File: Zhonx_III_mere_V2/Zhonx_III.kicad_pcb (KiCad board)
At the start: 2 copper layers, 70 x 97 mm, 133 parts, among them K1 L_Motor, K2 R_Motor, K3 USART, P1 JTAG, Q1 FDV301N, Q2 FDV301N, U1 MCP73213, U10 BSL214N, U11 BSL214N, U12 24LC64T, U14 STM32F405RGT6, U16 Line_1, U17 Line_2, U18 Line_3, U19 Line_4, U2 A3918, U20 Line_5, U3 A3918, U4 LTC2955CTS8-2, U5 SIB911DK, U6 SI1551DL, U7 LM2940, U8 MCP1700, U9 MCP1700, X1 16MHz

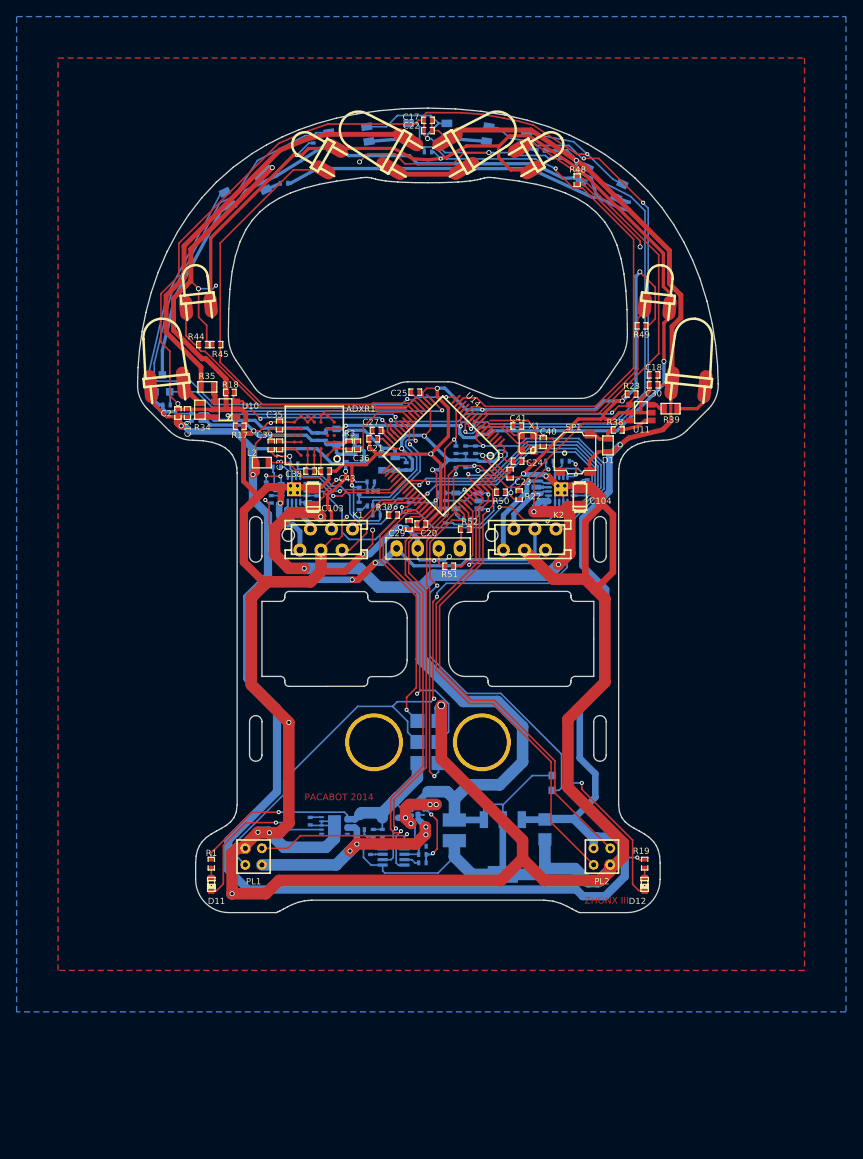
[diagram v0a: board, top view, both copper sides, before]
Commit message: Add ZHONX_III V2
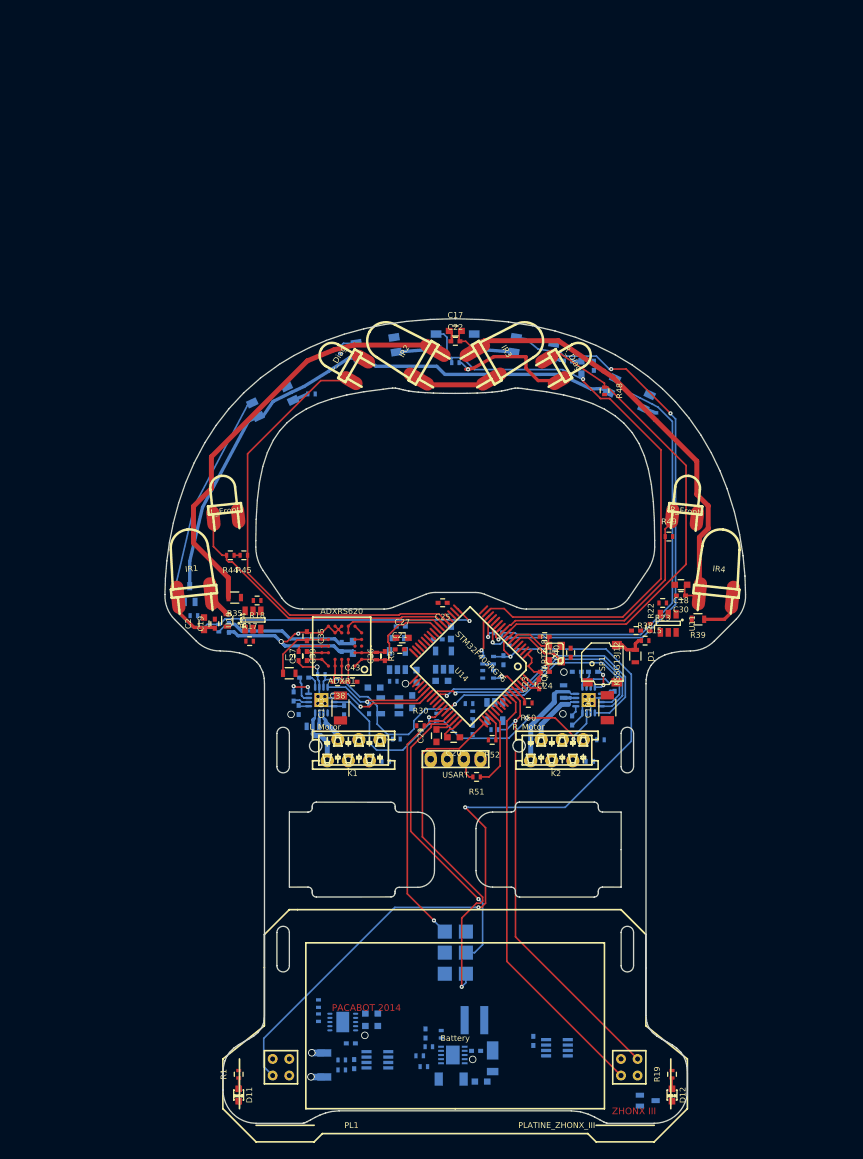
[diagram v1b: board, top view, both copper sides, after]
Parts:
- removed C100: 100uF, SM1210_Capa
- removed C101: 100uF, SM1206_Capa
- added C46: 2,2uF, Capacitors_SMD:C_0603, B.Cu at (111.0, 178.4)
- added C47: 330pF, Capacitors_SMD:C_0402, B.Cu at (104.3, 172.6)
- added C48: 0,47uF, Capacitors_SMD:C_0402, B.Cu at (110.4, 174.7)
- added C49: 0,47uF, Capacitors_SMD:C_0402, B.Cu at (101.3, 123.5)
- added C50: 0,47uF, Capacitors_SMD:C_0402, B.Cu at (105.8, 125.1)
- added C51: 0,47uF, Capacitors_SMD:C_0402, B.Cu at (97.5, 133.5)
- added C52: 10uF, Capacitors_SMD:C_0603, B.Cu at (101.1, 124.9)
- added C53: 10uF, Capacitors_SMD:C_0603, B.Cu at (107.4, 124.3)
- added C54: 10uF, Capacitors_SMD:C_0603, B.Cu at (98.1, 130.9)
- added C55: 33uF, Capacitors_SMD:C_1206, B.Cu at (107.4, 178.1)
- added L1: 2,2uH, ZHONX:XFL4020, B.Cu at (110.2, 171.0)
- added R36: 47K, Resistors_SMD:R_0402, B.Cu at (103.6, 175.3)
- added R37: 0.1 SHNT, Resistors_SMD:R_1206, B.Cu at (92.1, 176.4)
- added R40: 2,2K, Resistors_SMD:R_0402, B.Cu at (99.5, 139.8)
- added R41: 2,2K, Resistors_SMD:R_0402, B.Cu at (124.1, 139.8)
- added R42: 2,2K, Resistors_SMD:R_0402, B.Cu at (100.8, 137.1)
- added R43: 2,2K, Resistors_SMD:R_0402, B.Cu at (125.4, 137.2)
- ADXR1: footprint ADXRS620 -> ZHONX:ADXRS620
- C1, C17, C18, C2, C20, C26, C27, C29, C31, C9: footprint SM0402_ZHONX -> Capacitors_SMD:C_0603
- C10, C11, C12, C13, C14, C19, C21, C22, C23, C24, C25, C28, C3, C30, C32, C33, C35, C37, C38, C39, C4, C40, C41, C43, C44, C45, C5, C6, C7, C8: footprint SM0402_ZHONX -> Capacitors_SMD:C_0402
- C103, C104: footprint SM1206_Capa -> Capacitors_SMD:C_1206
- C15: value 0,1uF -> 10nF; footprint SM0402_ZHONX -> Capacitors_SMD:C_0402; moved to F.Cu
- C16: value 0,1uF -> 2,2uF; footprint SM0402_ZHONX -> Capacitors_SMD:C_0603
- C34: value 1uF -> 2.2uF; footprint SM0402_ZHONX -> Capacitors_SMD:C_0603
- C36: value 22nF -> 2,2nF; footprint SM0402_ZHONX -> Capacitors_SMD:C_0402
- C42: value 10uF -> 2.2uF; footprint SM0603_Capa -> Capacitors_SMD:C_0603
- D1: footprint SM0603 -> Resistors_SMD:R_0603
- D11: value Bleue -> BLUE; footprint LED-0603 -> ZHONX:LED-0603-DVB
- D12: value Blanc -> GREEN; footprint LED-0603 -> ZHONX:LED-0603-DVB
- IR1: footprint IR_LF -> ZHONX:IR_LF
- IR2: footprint IR_LD -> ZHONX:IR_LD
- IR3: footprint IR_RD -> ZHONX:IR_RD
- IR4: footprint IR_RF -> ZHONX:IR_RF
- K1, K2: footprint Connecteur_Moteur_Zhonx -> ZHONX:Connecteur_Moteur_Zhonx
- K3: footprint Conn_Serial_Zhonx -> ZHONX:Conn_Serial_Zhonx
- L2: value 10uH -> BEAD; footprint SM0603 -> Resistors_SMD:R_0603
- P1: footprint Zhonx_III_JTAG -> ZHONX:Zhonx_III_JTAG
- PL1: footprint Platine_Zhonx_III -> ZHONX:Platine_Zhonx_III
- Q1, Q2: value FDV301N -> BSS138; footprint SOT23GDS -> SMD_Packages:SOT-323
- R1: value 3,3K -> 620; footprint SM0402_ZHONX -> Resistors_SMD:R_0402
- R10, R11, R13, R14, R15, R17, R18, R2, R20, R21, R23, R24, R25, R26, R29, R30, R31, R32, R33, R44, R45, R48, R49, R50, R51, R52, R7, R8, R9: footprint SM0402_ZHONX -> Resistors_SMD:R_0402
- R12: value 100K -> 23,7K; footprint SM0402_ZHONX -> Resistors_SMD:R_0402
- R16: value 10K -> 47K; footprint SM0402_ZHONX -> Resistors_SMD:R_0402
- R19: value 820 -> 470; footprint SM0402_ZHONX -> Resistors_SMD:R_0402
- R22: value 47K -> 1M; footprint SM0402_ZHONX -> Resistors_SMD:R_0402
- R27, R28: value 0,2 -> 0,2 603; footprint SM0603_ZHONX -> Resistors_SMD:R_0603
- R3: value 90K -> 90.9K 1%; footprint SM0402_ZHONX -> Resistors_SMD:R_0402
- R34, R39: value 12 -> 10 1W; footprint SM0603_ZHONX -> Resistors_SMD:R_0603
- R35: value 2,8 -> 2,2 2W; footprint SM0603_ZHONX -> Resistors_SMD:R_0603
- R38: value 100 -> 0; footprint SM0402_ZHONX -> Resistors_SMD:R_0402
- R4: value 1M -> 10; footprint SM0402_ZHONX -> Resistors_SMD:R_0402
- R5: value 1M -> 6.2K; footprint SM0402_ZHONX -> Resistors_SMD:R_0402
- R58, R67: value 220 -> 82; footprint SM0402_ZHONX -> Resistors_SMD:R_0402
- R6: value 100K -> 10; footprint SM0402_ZHONX -> Resistors_SMD:R_0402
- R64: value 33 -> 22; footprint SM0402_ZHONX -> Resistors_SMD:R_0402
- SCH1: value BAT60 -> DFLS240; footprint SOD323 -> ZHONX:PowerDI-123
- SP1: footprint Buzzer_KSSG13J12 -> ZHONX:Buzzer_KSSG13J12
- U1: footprint MCP73213 -> ZHONX:MCP73213
- U10, U11: footprint SOT23_6 -> Housings_SOT-23_SOT-143_TSOT-6:SOT-23-6
- U12: footprint SOT23-5 -> Housings_SOT-23_SOT-143_TSOT-6:SOT-23-5
- U14: footprint TQFP_64 -> ZHONX:TQFP_64
- U16, U17, U18, U19, U20: footprint QRE1113GR -> ZHONX:QRE1113GR
- U2: value A3918 -> A3918_L; footprint QFN16_Termal_Pad -> ZHONX:QFN16_Termal_Pad
- U3: value A3918 -> A3918_R; footprint QFN16_Termal_Pad -> ZHONX:QFN16_Termal_Pad
- U4: value LTC2955CTS8-2 -> LTC2955CTS8-1; footprint LTC2955 -> ZHONX:LTC2955
- U5: value SIB911DK -> INA219; footprint SC75-6L -> ZHONX:LTC2955
- U6: value SI1551DL -> LT1761-5; footprint SC70 -> Housings_SOT-23_SOT-143_TSOT-6:SOT-23-5
- U7: value LM2940 -> LT1761-3.3; footprint SOT223 -> Housings_SOT-23_SOT-143_TSOT-6:SOT-23-5
- U8: value MCP1700 -> LT1761-3.3; footprint SOT23 -> Housings_SOT-23_SOT-143_TSOT-6:SOT-23-5
- U9: value MCP1700 -> LT3684; footprint SOT23 -> ZHONX:DFN-10
- X1: value 16MHz -> QUARTZ_8Z; footprint Quartz_8Z-16MHz -> ZHONX:Quartz_8Z-16MHz
- moved U9 75.7 mm to (107.6, 175.2), turned to 270 degrees
- moved R16 69.8 mm to (104.1, 176.6), turned to 0 degrees
- moved R4 67.0 mm to (94.2, 177.0)
- moved R15 65.7 mm to (104.7, 174.2), turned to 180 degrees
- moved R5 63.2 mm to (91.4, 169.0), turned to 270 degrees
- moved C15 40.7 mm to (129.7, 124.0), turned to 180 degrees
- moved Q2 39.7 mm to (131.1, 180.7)
- moved C14 35.2 mm to (95.7, 176.3), turned to 90 degrees
- moved SCH1 31.4 mm to (112.4, 175.5), turned to 90 degrees
- moved U5 30.7 mm to (98.5, 176.1), turned to 90 degrees
- moved U4 30.3 mm to (120.2, 174.7)
- moved C11 30.2 mm to (117.3, 173.5)
- moved C34 29.7 mm to (106.3, 130.1), turned to 180 degrees
- moved U8 29.4 mm to (100.0, 133.1), turned to 180 degrees
- moved C42 28.7 mm to (102.7, 132.6)
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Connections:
- net +5VA renamed +5VADC
- C10 pad 1: GND -> +3.3VADC
- C10 pad 2: N-000003 -> GND
- C14 pad 1: +8V -> Net-(C14-Pad1)
- C14 pad 2: GND -> Net-(C14-Pad2)
- C15 pad 1: +5V -> Net-(C15-Pad1)
- C15 pad 2: GND -> PIEZZO
- C16 pad 1: +3.3V -> +8V
- C17 pad 2: +5V -> +4.5V
- C18 pad 1: +5V -> +4.5V
- C19 pad 1: +5V -> +4.5V
- C2 pad 1: +5V -> +4.5V
- C22 pad 2: +5V -> +4.5V
- C30 pad 1: +5V -> +4.5V
- C31 pad 1: +5V -> +4.5V
- C32 pad 1: +5V -> +4.5V
- C34 pad 1: +5V -> GND
- C34 pad 2: GND -> +5V
- C42 pad 1: +3.3V -> GND
- C42 pad 2: GND -> +4.5V
- C9 pad 1: +BATT -> GND
- C9 pad 2: GND -> +8V
- D1 pad 2: +5V -> +4.5V
- D12 pad 2: N-0000059 -> Net-(D12-Pad2)
- IR1 pad 1: +5V -> +4.5V
- IR3 pad 1: +5V -> +4.5V
- IR4 pad 1: +5V -> +4.5V
- K1 pad 5: L_ENC_B -> Net-(K1-Pad5)
- K1 pad 6: L_ENC_A -> Net-(K1-Pad6)
- K2 pad 5: R_ENC_A -> Net-(K2-Pad5)
- K2 pad 6: R_ENC_B -> Net-(K2-Pad6)
- K3 pad 4: +5V -> +4.5V
- P1 pad 4: NSRST -> PA13/JTMS-SWO
- PL1 pad 5: +5V -> +4.5V
- PL1 pad 8: GND -> WKUP
- R11 pad 2: N-00000103 -> Net-(R11-Pad2)
- R12 pad 1: N-000005 -> Net-(R12-Pad1)
- R12 pad 2: N-0000012 -> GND
- R15 pad 1: TEST_BAT -> Net-(R15-Pad1)
- R15 pad 2: N-0000093 -> Net-(C47-Pad1)
- R16 pad 1: GND -> Net-(R16-Pad1)
- R16 pad 2: TEST_BAT -> +4.5V
- R19 pad 2: +5V -> +4.5V
- R22 pad 1: PIEZZO -> Net-(C15-Pad1)
- R4 pad 1: GND -> Net-(C14-Pad1)
- R4 pad 2: GET_BAT_ADC -> +BATT
- R5 pad 1: +8V -> FAST_CHARGE
- R5 pad 2: N-0000067 -> Net-(R11-Pad2)
- R58 pad 2: +5V -> +4.5V
- R6 pad 1: +9V -> Net-(C14-Pad2)
- R6 pad 2: GND -> +8V
- R64 pad 2: +5V -> +4.5V
- R67 pad 2: +5V -> +4.5V
- R9 pad 1: N-000003 -> EN_PW_ADC
- R9 pad 2: N-000005 -> GND
- SCH1 pad 1: +9V -> GND
- SCH1 pad 2: N-000003 -> Net-(C48-Pad1)
- SP1 pad 1: +5V -> +4.5V
- U1 pad 10: N-00000103 -> Net-(R11-Pad2)
- U1 pad 3: +BATT -> +8V
- U1 pad 4: +BATT -> +8V
- U11 pad 3: PIEZZO -> Net-(C15-Pad1)
- U14 pad 16: Enable_IR_Line -> Line_IR_L1
- U14 pad 2: (no net) -> PW_LED
- U14 pad 20: Line_IR_L1 -> (no net)
- U14 pad 25: TEST_BAT -> (no net)
- U14 pad 26: GET_BAT_ADC -> (no net)
- U14 pad 28: (no net) -> Enable_IR_Line
- U14 pad 50: PW_LED -> FAST_CHARGE
- U14 pad 53: (no net) -> WP_EEPROM
- U14 pad 55: WP_EEPROM -> PA13/JTMS-SWO
- U16 pad 2: N-0000074 -> Net-(Q1-Pad3)
- U17 pad 2: N-0000074 -> Net-(Q1-Pad3)
- U20 pad 2: N-0000074 -> Net-(Q1-Pad3)
- U4 pad 6: N-000003 -> +8V
- U4 pad 7: N-0000012 -> EN_DC/DC
- U5 pad 1: N-000003 -> Net-(C14-Pad1)
- U5 pad 2: N-000005 -> Net-(C14-Pad2)
- U5 pad 3: +BATT -> GND
- U5 pad 4: N-000003 -> +3.3VADC
- U5 pad 5: +9V -> I2C_SCL
- U5 pad 6: +8V -> I2C_SDA
- U6 pad 1: GND -> +8V
- U6 pad 2: GET_BAT_ADC -> GND
- U6 pad 3: N-0000093 -> EN_PW_ADC
- U6 pad 4: +8V -> Net-(C49-Pad1)
- U6 pad 5: N-0000067 -> +5V
- U7 pad 1: +8V -> +5V
- U7 pad 4: GND -> Net-(C50-Pad1)
- U8 pad 1: GND -> +4.5V
- U8 pad 2: +3.3V -> GND
- U8 pad 3: +5V -> +4.5V
- U9 pad 1: GND -> +4.5V
- U9 pad 2: +3.3VADC -> Net-(C48-Pad2)
- U9 pad 3: +5V -> Net-(C48-Pad1)
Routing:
- net GND: track 838.5 -> 52.8 mm, vias 35 -> 3
- net +5V: track 403.8 -> 8.52 mm, vias 8 -> 0
- net +3.3VADC: track 169.6 -> 39.3 mm, vias 5 -> 2
- net Line_IR_L1: track 73.7 -> 2.06 mm, vias 1 -> 0
- net N-0000074: track 68.6 -> 0.00 mm
- net Net-(Q1-Pad3): track 0.00 -> 68.6 mm
- net +4.5V: track 0.00 -> 65.1 mm
- net WKUP: track 65.3 -> 5.91 mm, vias 2 -> 1
- net POWER_KILL: track 60.3 -> 3.75 mm, vias 2 -> 1
- net +3.3V: track 67.2 -> 12.7 mm, vias 6 -> 0
- net PW_LED: track 52.7 -> 0.00 mm, vias 2 -> 0
- net +9V: track 40.1 -> 0.00 mm, vias 1 -> 0
- net Enable_IR_Line: track 37.6 -> 0.00 mm, vias 1 -> 0
- net RFront_TX: track 34.5 -> 0.77 mm, vias 2 -> 0
- net +BATT: track 37.2 -> 4.30 mm, vias 4 -> 1
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- removed copper zone on B.Cu, net GND
- removed copper zone on F.Cu, net GND
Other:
- copper layers 2 -> 4
- net class Default: via_drill 0.3 -> 0.2
- rule via_min_drill: 0.3 -> 0.2
